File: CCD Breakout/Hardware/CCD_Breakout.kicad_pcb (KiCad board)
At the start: 2 copper layers, 9 parts, among them J1 Conn_01x03_Pin, U1 ILX511

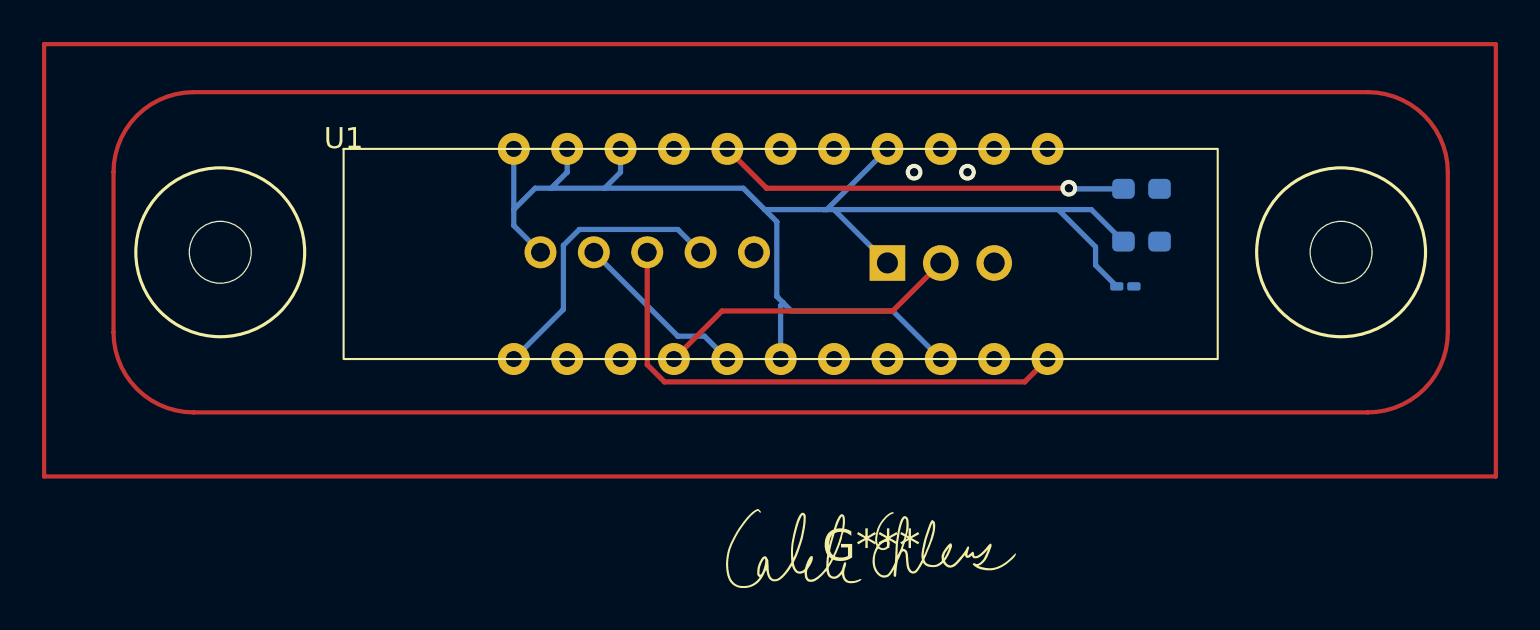
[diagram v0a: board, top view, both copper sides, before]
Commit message: finish ccd board
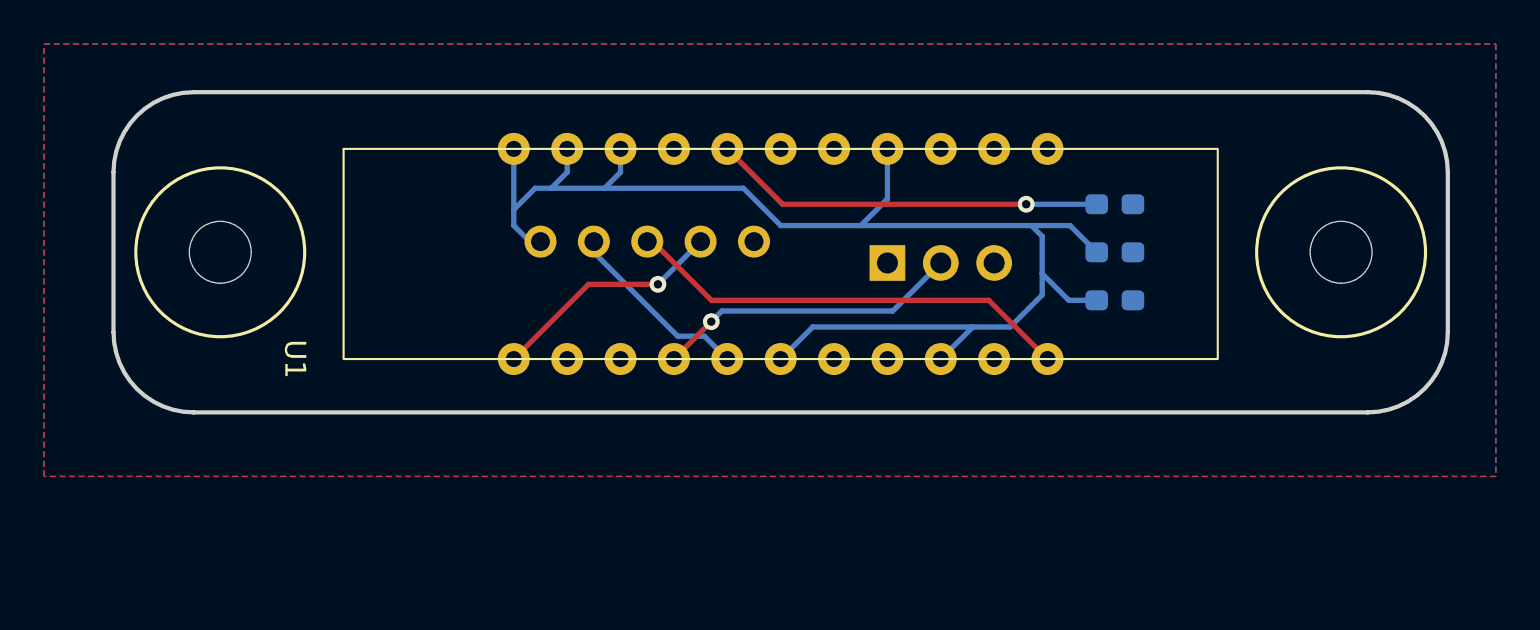
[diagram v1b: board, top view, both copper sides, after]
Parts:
- C3: footprint Capacitor_SMD:C_0201_0603Metric_Pad0.64x0.40mm_HandSolder -> Capacitor_SMD:C_0603_1608Metric_Pad1.08x0.95mm_HandSolder
- G***: moved to B.Cu
- moved G*** 21.1 mm to (88.4, 26.9), turned to -90 degrees
- moved C2 3.07 mm to (84.2, 29.2)
- moved C3 1.70 mm to (84.2, 26.9)
- moved C1 1.47 mm to (84.2, 24.6)
- moved Conn1 0.51 mm to (56.9, 26.4)
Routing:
- net øROG: track 25.2 -> 21.4 mm
- net +5V: track 69.1 -> 65.9 mm
- net Vout: track 13.7 -> 11.2 mm, vias 0 -> 1
- net Net-(U1-VGG): track 19.6 -> 18.7 mm
- net SHSW: vias 0 -> 1
- net GND: vias 2 -> 0
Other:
- board outline added: 63.5 x 15.2 mm
- board text added: "CCD Breakout"
